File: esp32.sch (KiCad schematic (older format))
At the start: 32 parts, among them J10 Conn_01x01, J11 Conn_01x04, J12 Conn_01x01, J13 Conn_01x01, J15 Conn_01x01, J16 Conn_01x01, J17 Conn_01x01, J18 Conn_01x02, J19 Conn_01x01, J25 Conn_01x01, J26 Conn_01x02, J6 Conn_01x04, J7 Conn_01x04, J8 Conn_01x04, J9 Conn_01x01, Q1 2N7002, U2 ESP32-DEVKITC

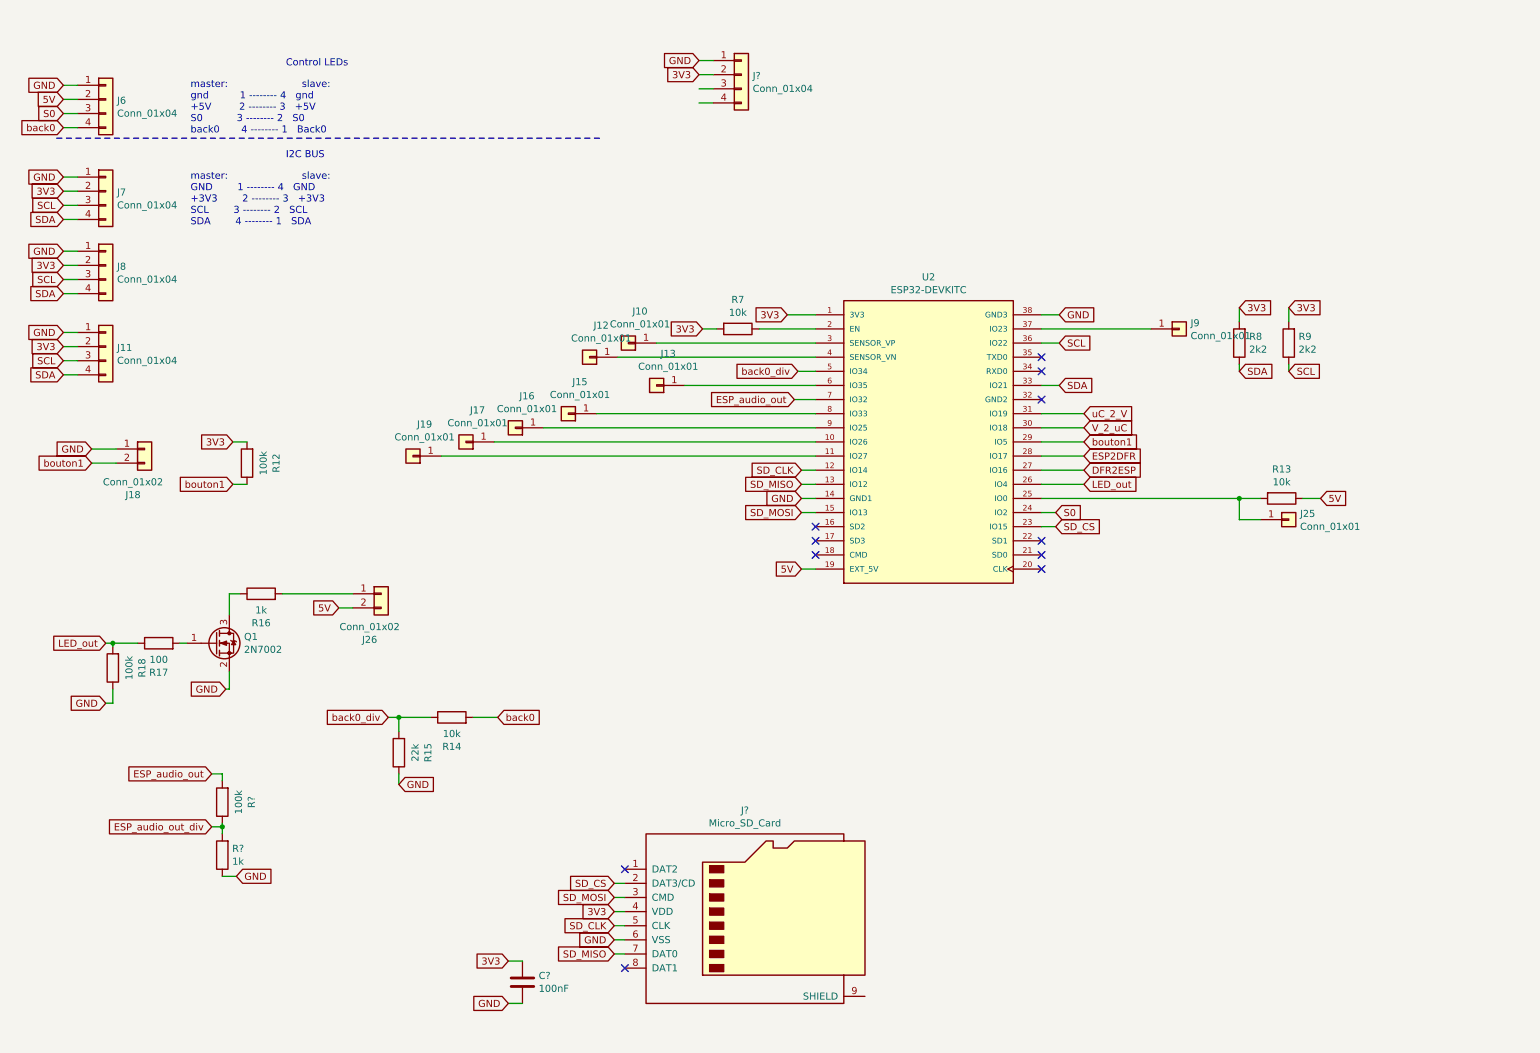
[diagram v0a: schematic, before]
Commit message: maj
simplification dfr
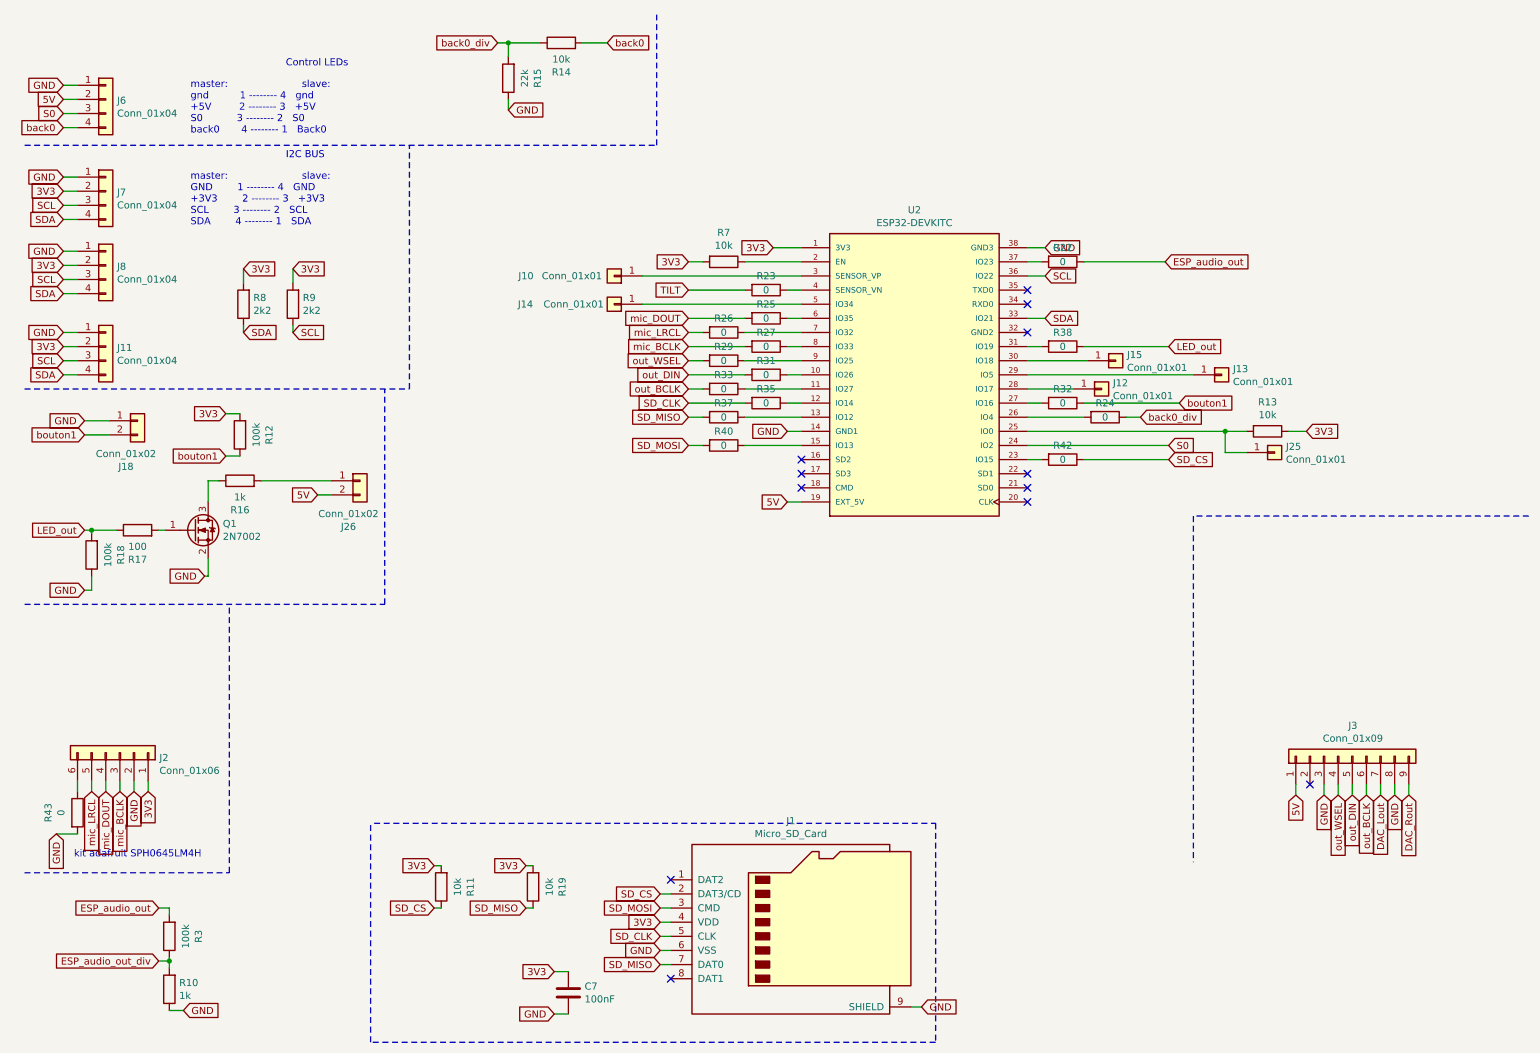
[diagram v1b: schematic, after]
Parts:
- removed J16, J17, J19, J9: Conn_01x01, Connector_PinHeader_2.54mm:PinHeader_1x01_P2.54mm_Vertical, symbol Connector_Generic:Conn_01x01
- removed J?: Conn_01x04, Connector_JST:JST_XH_B4B-XH-A_1x04_P2.50mm_Vertical, symbol Connector_Generic:Conn_01x04
- added J14: Conn_01x01, Connector_PinHeader_2.54mm:PinHeader_1x01_P2.54mm_Vertical, symbol Connector_Generic:Conn_01x01
- added J2: Conn_01x06, Connector_PinSocket_2.54mm:PinSocket_1x06_P2.54mm_Vertical, symbol Connector_Generic:Conn_01x06
- added J3: Conn_01x09, Connector_PinSocket_2.54mm:PinSocket_1x09_P2.54mm_Vertical, symbol Connector_Generic:Conn_01x09
- added R11, R19: 10k, Resistor_SMD:R_0603_1608Metric_Pad1.05x0.95mm_HandSolder, symbol Device:R
- added R22, R23, R24, R25, R26, R27, R29, R31, R32, R33, R35, R37, R38, R40, R42, R43: 0, Resistor_SMD:R_0603_1608Metric_Pad1.05x0.95mm_HandSolder, symbol Device:R
- J1: renamed from J?; footprint (none) -> Connector_Card:microSD_HC_Molex_104031-0811
- gave numbers to parts that had none: 3
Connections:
- net ESP2DFR is gone; now on an unnamed net: U2.28 (IO17)
- net V_2_uC is gone; now on an unnamed net: U2.30 (IO18)
- net 3V3: now also R13.1, J2.1 (Pin_1), R11.2, R19.2
- net 5V: now also J3.1 (Pin_1); no longer R13.1
- net ESP_audio_out: now also R22.1; no longer U2.7 (IO32)
- net GND: now also J1.9 (SHIELD), J2.2 (Pin_2), J3.3 (Pin_3), J3.8 (Pin_8), R43.2
- net LED_out: now also R38.1; no longer U2.26 (IO4)
- net SD_CLK: now also R35.2; no longer U2.12 (IO14)
- net SD_CS: now also R11.1, R42.1; no longer U2.23 (IO15)
- net SD_MISO: now also R19.1, R37.2; no longer U2.13 (IO12)
- net SD_MOSI: now also R40.2; no longer U2.15 (IO13)
- net back0_div: now also R24.1; no longer U2.5 (IO34)
- net bouton1: now also R32.1; no longer U2.29 (IO5)
- net at U2.10 (IO26): now also R31.1
- net at U2.11 (IO27): now also R33.1
- net at U2.37 (IO23): now also R22.2
- net at J12.1 (Pin_1): no longer U2.4 (SENSOR_VN)
- net at J13.1 (Pin_1): now also U2.29 (IO5); no longer U2.6 (IO35)
- net at J15.1 (Pin_1): no longer U2.8 (IO33)
- net at U2.9 (IO25): now also R29.1
- net DFR2ESP: no longer names the net of U2.27 (IO16)
- net DFR2ESP: now also R32.2
- net uC_2_V: no longer names the net of U2.31 (IO19)
- net uC_2_V: now also R38.2
- new net: R35.1, U2.12 (IO14)
- new net: R37.1, U2.13 (IO12)
- new net: R40.1, U2.15 (IO13)
- new net: R42.2, U2.23 (IO15)
- new net: R24.2, U2.26 (IO4)
- new net: R23.1, U2.4 (SENSOR_VN)
- new net: J14.1 (Pin_1), U2.5 (IO34)
- new net: R25.1, U2.6 (IO35)
- new net: R26.1, U2.7 (IO32)
- new net: R27.1, U2.8 (IO33)
- new net: J2.6 (Pin_6), R43.1
- new net DAC_Lout: J3.7 (Pin_7)
- new net DAC_Rout: J3.9 (Pin_9)
- new net TILT: R23.2
- new net mic_BCLK: J2.3 (Pin_3), R27.2
- new net mic_DOUT: J2.4 (Pin_4), R25.2
- new net mic_LRCL: J2.5 (Pin_5), R26.2
- new net out_BCLK: J3.6 (Pin_6), R33.2
- new net out_DIN: J3.5 (Pin_5), R31.2
- new net out_WSEL: J3.4 (Pin_4), R29.2
- no-connect marks 11 -> 12
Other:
- note added: "kit adafruit SPH0645LM4H"
- moved on the sheet: C7, J1, J10, J18, J25, J26, Q1, R10, R12, R13, R14, R15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
